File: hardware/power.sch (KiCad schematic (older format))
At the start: 12 parts, among them Q4 PMOS-DMG3413L, U18 AZ1117E, U4 MCP73831T

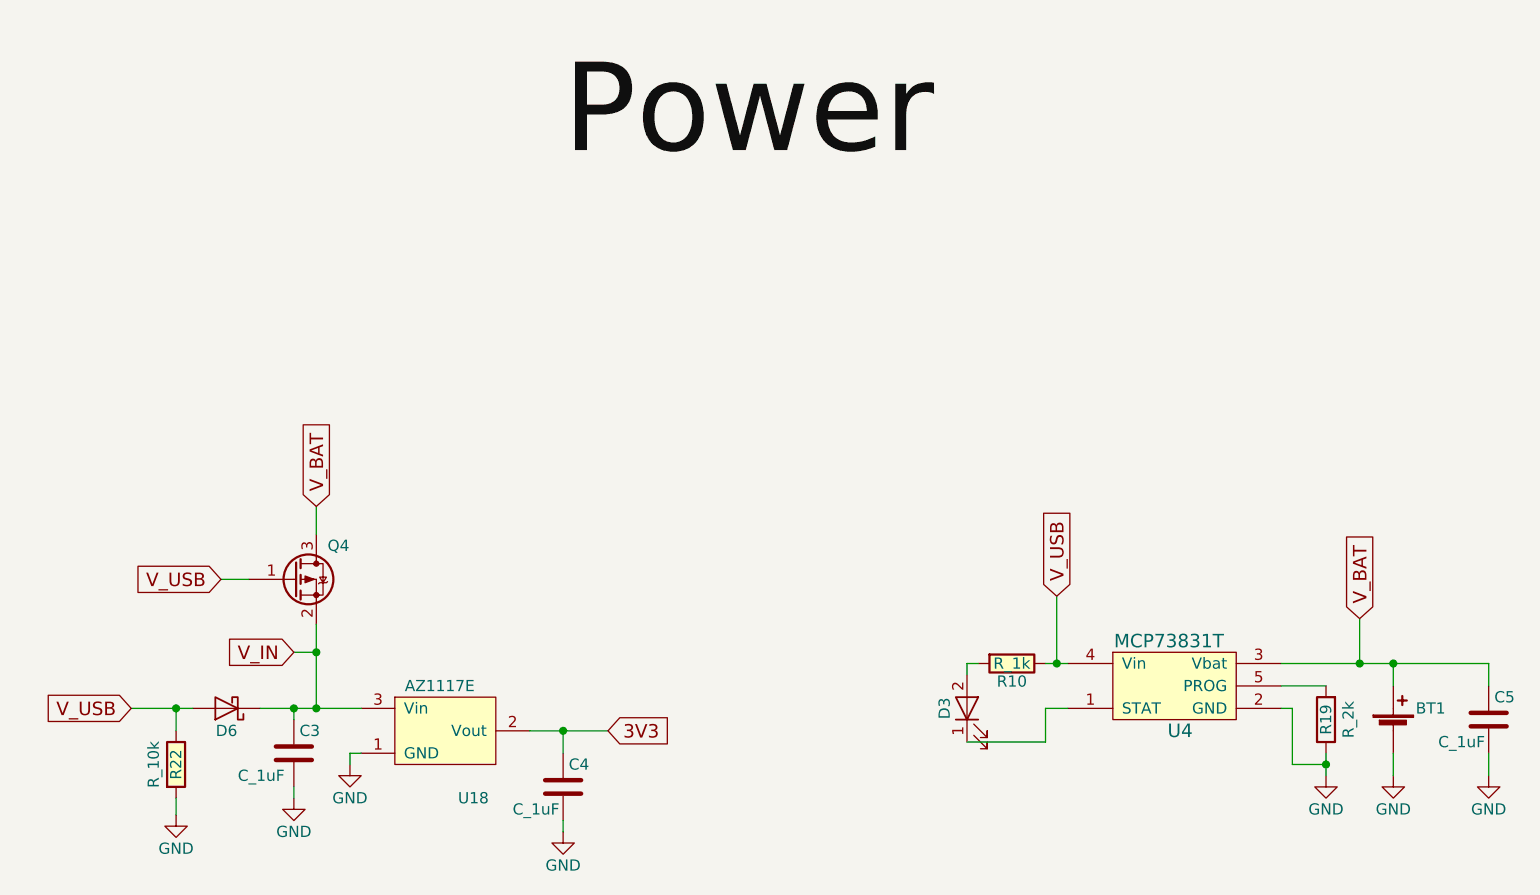
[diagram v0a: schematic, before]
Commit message: update
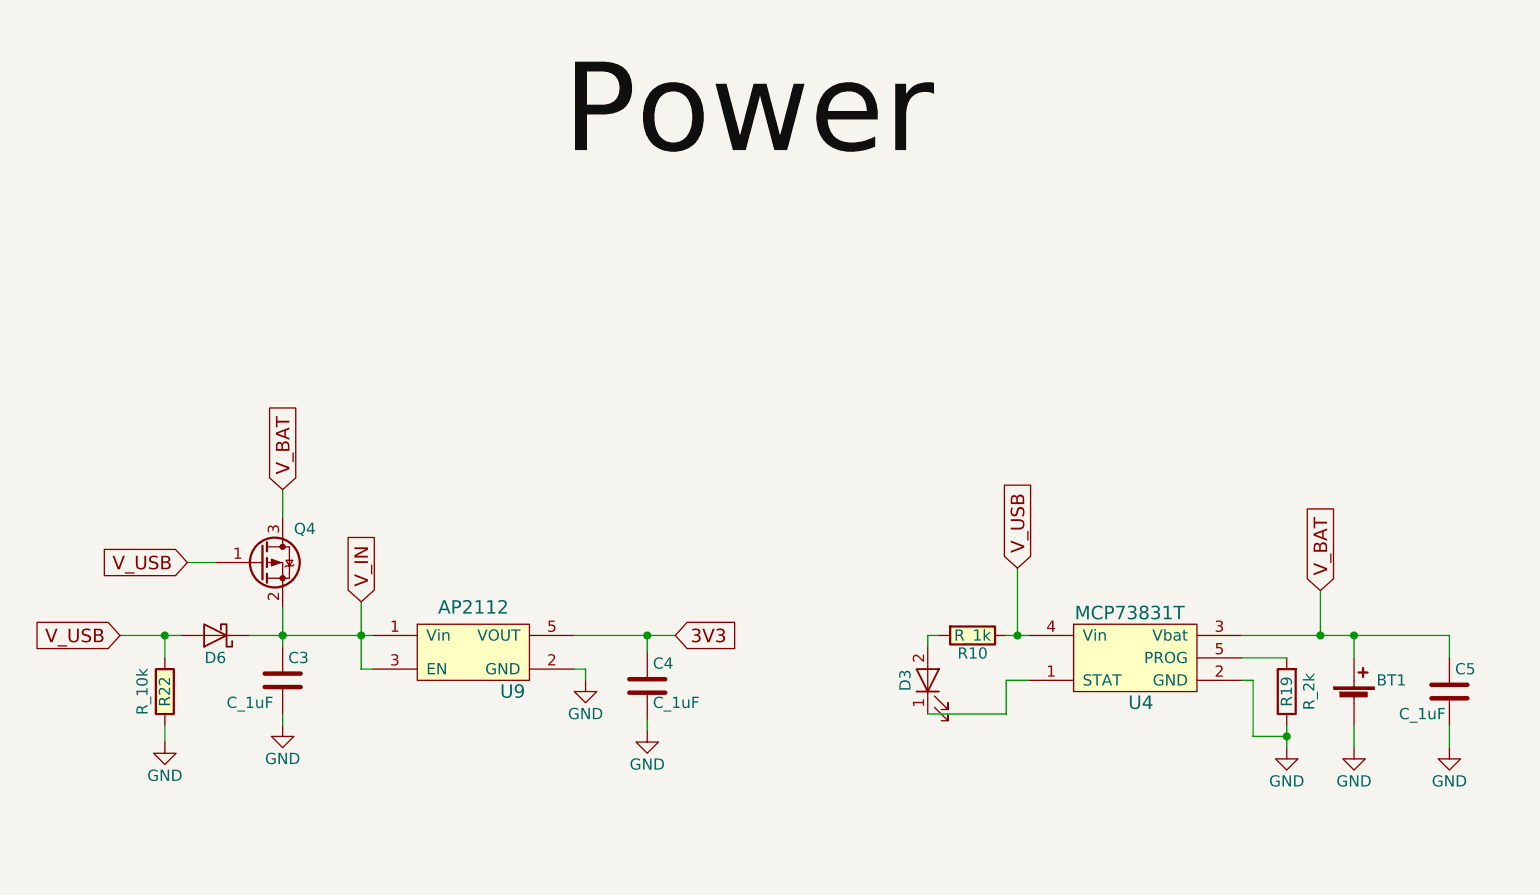
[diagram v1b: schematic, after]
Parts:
- removed U18: AZ1117E, open-automation:SPX1117M3, symbol AZ1117E
- added U9: AP2112, TO_SOT_Packages_SMD:SOT-23-5, symbol AP2112
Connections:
- net 3V3: now also U9.5 (VOUT)
- net GND: now also U9.2 (GND)
- net V_IN: now also U9.1 (Vin), U9.3 (EN)
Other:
- moved on the sheet: BT1, C3, C4, C5, D3, D6, Q4, R10, R19, R22, U4
